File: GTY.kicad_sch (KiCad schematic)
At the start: 2 parts, among them J5 DF40HC(3.0)-120DS, U1 XCKU5P-FFVB676

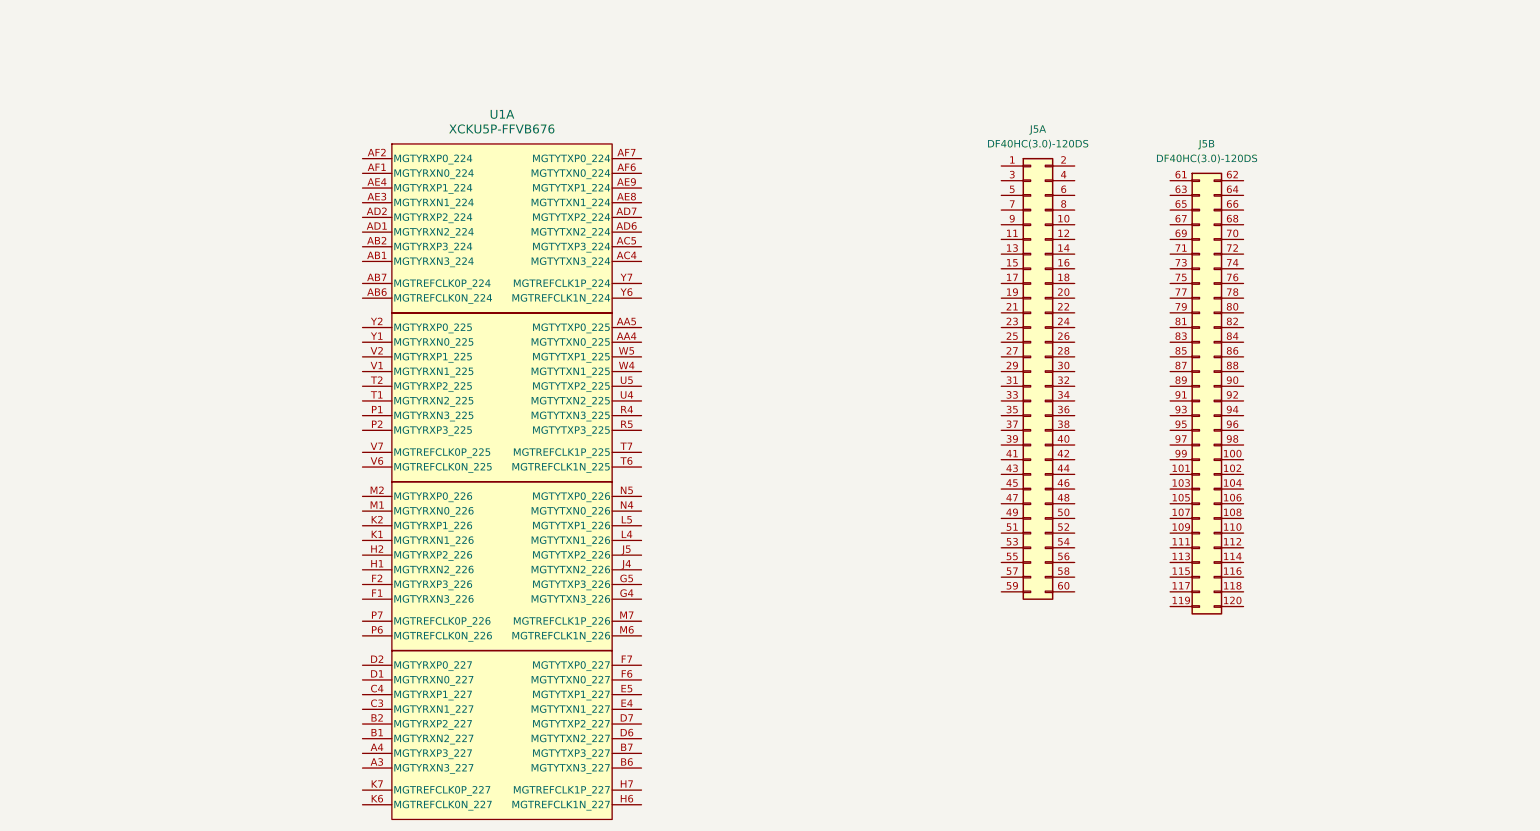
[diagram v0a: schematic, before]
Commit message: finishing schematic
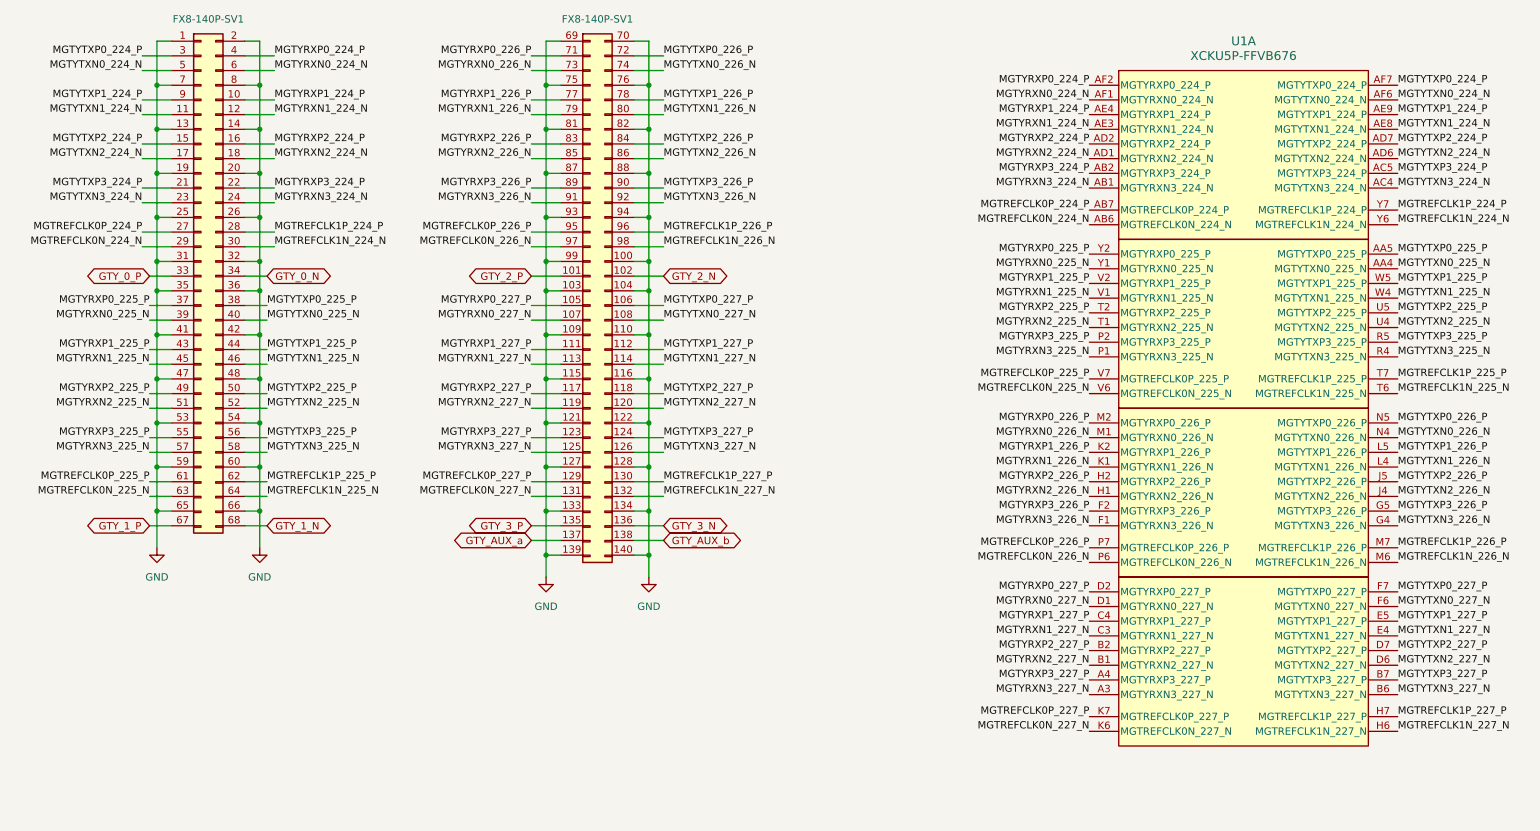
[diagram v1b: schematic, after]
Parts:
- J5: value DF40HC(3.0)-120DS -> FX8-140P-SV1; symbol dfdtc_Connector:Conn_02x60_Odd_Even -> dfdtc_Connector:Conn_02x70_Odd_Even
- J5: value DF40HC(3.0)-120DS -> FX8-140P-SV1; footprint Connector_Hirose_DF40:Hirose_DF40C-120DS-0.4V_2x60_P0.4mm -> Connector_Hirose_FX8:Hirose_FX8-140P-SV_2x70_P0.6mm; symbol dfdtc_Connector:Conn_02x60_Odd_Even -> dfdtc_Connector:Conn_02x70_Odd_Even
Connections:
- net GND: now reaches J5.100 (Pin_100)
- net GND: now also J5.1 (Pin_1), J5.103 (Pin_103), J5.104 (Pin_104), J5.109 (Pin_109), J5.110 (Pin_110), J5.115 (Pin_115), J5.116 (Pin_116), J5.121, J5.122, J5.127, J5.128, J5.13 (Pin_13), J5.133, J5.134, J5.139, J5.14 (Pin_14), J5.140, J5.19 (Pin_19), J5.2 (Pin_2), J5.20 (Pin_20), J5.25 (Pin_25), J5.26 (Pin_26), J5.31 (Pin_31), J5.32 (Pin_32), J5.35 (Pin_35), J5.36 (Pin_36), J5.41 (Pin_41), J5.42 (Pin_42), J5.47 (Pin_47), J5.48 (Pin_48), J5.53 (Pin_53), J5.54 (Pin_54), J5.59 (Pin_59), J5.60 (Pin_60), J5.65 (Pin_65), J5.66 (Pin_66), J5.69 (Pin_69), J5.7 (Pin_7), J5.70 (Pin_70), J5.75 (Pin_75), J5.76 (Pin_76), J5.8 (Pin_8), J5.81 (Pin_81), J5.82 (Pin_82), J5.87 (Pin_87), J5.88 (Pin_88), J5.93 (Pin_93), J5.94 (Pin_94), J5.99 (Pin_99)
- net GTY_2_P: now reaches J5.101 (Pin_101)
- net GTY_2_N: now reaches J5.102 (Pin_102)
- net MGTYRXP0_227_P: now reaches J5.105 (Pin_105)
- net MGTYRXP0_227_P: now also U1.D2 (MGTYRXP0_227_P)
- net MGTYTXP0_227_P: now reaches J5.106 (Pin_106)
- net MGTYTXP0_227_P: now also U1.F7 (MGTYTXP0_227_P)
- net MGTYRXN0_227_N: now reaches J5.107 (Pin_107)
- net MGTYRXN0_227_N: now also U1.D1 (MGTYRXN0_227_N)
- net MGTYTXN0_227_N: now reaches J5.108 (Pin_108)
- net MGTYTXN0_227_N: now also U1.F6 (MGTYTXN0_227_N)
- net MGTYRXP1_227_P: now reaches J5.111 (Pin_111)
- net MGTYRXP1_227_P: now also U1.C4 (MGTYRXP1_227_P)
- net MGTYTXP1_227_P: now reaches J5.112 (Pin_112)
- net MGTYTXP1_227_P: now also U1.E5 (MGTYTXP1_227_P)
- net MGTYRXN1_227_N: now reaches J5.113 (Pin_113)
- net MGTYRXN1_227_N: now also U1.C3 (MGTYRXN1_227_N)
- net MGTYTXN1_227_N: now reaches J5.114 (Pin_114)
- net MGTYTXN1_227_N: now also U1.E4 (MGTYTXN1_227_N)
- net MGTYRXP2_227_P: now reaches J5.117 (Pin_117)
- net MGTYRXP2_227_P: now also U1.B2 (MGTYRXP2_227_P)
- net MGTYTXP2_227_P: now reaches J5.118 (Pin_118)
- net MGTYTXP2_227_P: now also U1.D7 (MGTYTXP2_227_P)
- net MGTYRXN2_227_N: now reaches J5.119 (Pin_119)
- net MGTYRXN2_227_N: now also U1.B1 (MGTYRXN2_227_N)
- net MGTYTXN2_227_N: now reaches J5.120 (Pin_120)
- net MGTYTXN2_227_N: now also U1.D6 (MGTYTXN2_227_N)
- net MGTYRXP0_226_P: now reaches J5.71 (Pin_71)
- net MGTYRXP0_226_P: now also U1.M2 (MGTYRXP0_226_P)
- net MGTYTXP0_226_P: now reaches J5.72 (Pin_72)
- net MGTYTXP0_226_P: now also U1.N5 (MGTYTXP0_226_P)
- net MGTYRXN0_226_N: now reaches J5.73 (Pin_73)
- net MGTYRXN0_226_N: now also U1.M1 (MGTYRXN0_226_N)
- net MGTYTXN0_226_N: now reaches J5.74 (Pin_74)
- net MGTYTXN0_226_N: now also U1.N4 (MGTYTXN0_226_N)
- net MGTYRXP1_226_P: now reaches J5.77 (Pin_77)
- net MGTYRXP1_226_P: now also U1.K2 (MGTYRXP1_226_P)
- net MGTYTXP1_226_P: now reaches J5.78 (Pin_78)
- net MGTYTXP1_226_P: now also U1.L5 (MGTYTXP1_226_P)
- net MGTYRXN1_226_N: now reaches J5.79 (Pin_79)
- net MGTYRXN1_226_N: now also U1.K1 (MGTYRXN1_226_N)
- net MGTYTXN1_226_N: now reaches J5.80 (Pin_80)
- net MGTYTXN1_226_N: now also U1.L4 (MGTYTXN1_226_N)
- net MGTYRXP2_226_P: now reaches J5.83 (Pin_83)
- net MGTYRXP2_226_P: now also U1.H2 (MGTYRXP2_226_P)
- net MGTYTXP2_226_P: now reaches J5.84 (Pin_84)
- net MGTYTXP2_226_P: now also U1.J5 (MGTYTXP2_226_P)
- net MGTYRXN2_226_N: now reaches J5.85 (Pin_85)
- net MGTYRXN2_226_N: now also U1.H1 (MGTYRXN2_226_N)
- net MGTYTXN2_226_N: now reaches J5.86 (Pin_86)
- net MGTYTXN2_226_N: now also U1.J4 (MGTYTXN2_226_N)
- net MGTYRXP3_226_P: now reaches J5.89 (Pin_89)
- net MGTYRXP3_226_P: now also U1.F2 (MGTYRXP3_226_P)
- net MGTYTXP3_226_P: now reaches J5.90 (Pin_90)
- net MGTYTXP3_226_P: now also U1.G5 (MGTYTXP3_226_P)
- net MGTYRXN3_226_N: now reaches J5.91 (Pin_91)
- net MGTYRXN3_226_N: now also U1.F1 (MGTYRXN3_226_N)
- net MGTYTXN3_226_N: now reaches J5.92 (Pin_92)
- net MGTYTXN3_226_N: now also U1.G4 (MGTYTXN3_226_N)
- net MGTREFCLK0P_226_P: now reaches J5.95 (Pin_95)
- net MGTREFCLK0P_226_P: now also U1.P7 (MGTREFCLK0P_226_P)
- net MGTREFCLK1P_226_P: now reaches J5.96 (Pin_96)
- net MGTREFCLK1P_226_P: now also U1.M7 (MGTREFCLK1P_226_P)
- net MGTREFCLK0N_226_N: now reaches J5.97 (Pin_97)
- net MGTREFCLK0N_226_N: now also U1.P6 (MGTREFCLK0N_226_N)
- net MGTREFCLK1N_226_N: now reaches J5.98 (Pin_98)
- net MGTREFCLK1N_226_N: now also U1.M6 (MGTREFCLK1N_226_N)
- net MGTYRXP1_224_P: now reaches J5.10 (Pin_10)
- net MGTYRXP1_224_P: now also U1.AE4 (MGTYRXP1_224_P)
- net MGTYTXN1_224_N: now reaches J5.11 (Pin_11)
- net MGTYTXN1_224_N: now also U1.AE8 (MGTYTXN1_224_N)
- net MGTYRXN1_224_N: now reaches J5.12 (Pin_12)
- net MGTYRXN1_224_N: now also U1.AE3 (MGTYRXN1_224_N)
- net MGTYTXP2_224_P: now reaches J5.15 (Pin_15)
- net MGTYTXP2_224_P: now also U1.AD7 (MGTYTXP2_224_P)
- net MGTYRXP2_224_P: now reaches J5.16 (Pin_16)
- net MGTYRXP2_224_P: now also U1.AD2 (MGTYRXP2_224_P)
- net MGTYTXN2_224_N: now reaches J5.17 (Pin_17)
- net MGTYTXN2_224_N: now also U1.AD6 (MGTYTXN2_224_N)
- net MGTYRXN2_224_N: now reaches J5.18 (Pin_18)
- net MGTYRXN2_224_N: now also U1.AD1 (MGTYRXN2_224_N)
- net MGTYTXP3_224_P: now reaches J5.21 (Pin_21)
- net MGTYTXP3_224_P: now also U1.AC5 (MGTYTXP3_224_P)
- net MGTYRXP3_224_P: now reaches J5.22 (Pin_22)
- net MGTYRXP3_224_P: now also U1.AB2 (MGTYRXP3_224_P)
- net MGTYTXN3_224_N: now reaches J5.23 (Pin_23)
- net MGTYTXN3_224_N: now also U1.AC4 (MGTYTXN3_224_N)
- net MGTYRXN3_224_N: now reaches J5.24 (Pin_24)
- net MGTYRXN3_224_N: now also U1.AB1 (MGTYRXN3_224_N)
- net MGTREFCLK0P_224_P: now reaches J5.27 (Pin_27)
- net MGTREFCLK0P_224_P: now also U1.AB7 (MGTREFCLK0P_224_P)
- net MGTREFCLK1P_224_P: now reaches J5.28 (Pin_28)
- net MGTREFCLK1P_224_P: now also U1.Y7 (MGTREFCLK1P_224_P)
- net MGTREFCLK0N_224_N: now reaches J5.29 (Pin_29)
- net MGTREFCLK0N_224_N: now also U1.AB6 (MGTREFCLK0N_224_N)
- net MGTYTXP0_224_P: now reaches J5.3 (Pin_3)
- net MGTYTXP0_224_P: now also U1.AF7 (MGTYTXP0_224_P)
- net MGTREFCLK1N_224_N: now reaches J5.30 (Pin_30)
- net MGTREFCLK1N_224_N: now also U1.Y6 (MGTREFCLK1N_224_N)
- net GTY_0_P: now reaches J5.33 (Pin_33)
- net GTY_0_N: now reaches J5.34 (Pin_34)
- net MGTYRXP0_225_P: now reaches J5.37 (Pin_37)
- net MGTYRXP0_225_P: now also U1.Y2 (MGTYRXP0_225_P)
- net MGTYTXP0_225_P: now reaches J5.38 (Pin_38)
- net MGTYTXP0_225_P: now also U1.AA5 (MGTYTXP0_225_P)
- net MGTYRXN0_225_N: now reaches J5.39 (Pin_39)
- net MGTYRXN0_225_N: now also U1.Y1 (MGTYRXN0_225_N)
- net MGTYRXP0_224_P: now reaches J5.4 (Pin_4)
- net MGTYRXP0_224_P: now also U1.AF2 (MGTYRXP0_224_P)
- net MGTYTXN0_225_N: now reaches J5.40 (Pin_40)
- net MGTYTXN0_225_N: now also U1.AA4 (MGTYTXN0_225_N)
- net MGTYRXP1_225_P: now reaches J5.43 (Pin_43)
- net MGTYRXP1_225_P: now also U1.V2 (MGTYRXP1_225_P)
- net MGTYTXP1_225_P: now reaches J5.44 (Pin_44)
- net MGTYTXP1_225_P: now also U1.W5 (MGTYTXP1_225_P)
- net MGTYRXN1_225_N: now reaches J5.45 (Pin_45)
- net MGTYRXN1_225_N: now also U1.V1 (MGTYRXN1_225_N)
- net MGTYTXN1_225_N: now reaches J5.46 (Pin_46)
- net MGTYTXN1_225_N: now also U1.W4 (MGTYTXN1_225_N)
- net MGTYRXP2_225_P: now reaches J5.49 (Pin_49)
- net MGTYRXP2_225_P: now also U1.T2 (MGTYRXP2_225_P)
- net MGTYTXN0_224_N: now reaches J5.5 (Pin_5)
- net MGTYTXN0_224_N: now also U1.AF6 (MGTYTXN0_224_N)
- net MGTYTXP2_225_P: now reaches J5.50 (Pin_50)
- net MGTYTXP2_225_P: now also U1.U5 (MGTYTXP2_225_P)
- net MGTYRXN2_225_N: now reaches J5.51 (Pin_51)
- net MGTYRXN2_225_N: now also U1.T1 (MGTYRXN2_225_N)
- net MGTYTXN2_225_N: now reaches J5.52 (Pin_52)
- net MGTYTXN2_225_N: now also U1.U4 (MGTYTXN2_225_N)
- net MGTYRXP3_225_P: now reaches J5.55 (Pin_55)
- net MGTYRXP3_225_P: now also U1.P2 (MGTYRXP3_225_P)
- net MGTYTXP3_225_P: now reaches J5.56 (Pin_56)
- net MGTYTXP3_225_P: now also U1.R5 (MGTYTXP3_225_P)
- net MGTYRXN3_225_N: now reaches J5.57 (Pin_57)
- net MGTYRXN3_225_N: now also U1.P1 (MGTYRXN3_225_N)
- net MGTYTXN3_225_N: now reaches J5.58 (Pin_58)
- net MGTYTXN3_225_N: now also U1.R4 (MGTYTXN3_225_N)
- net MGTYRXN0_224_N: now reaches J5.6 (Pin_6)
- net MGTYRXN0_224_N: now also U1.AF1 (MGTYRXN0_224_N)
- net MGTYTXP1_224_P: now reaches J5.9 (Pin_9)
- net MGTYTXP1_224_P: now also U1.AE9 (MGTYTXP1_224_P)
- net MGTYRXN3_227_N: now reaches U1.A3 (MGTYRXN3_227_N)
- net MGTYRXN3_227_N: now also J5.125
- net MGTYRXP3_227_P: now reaches U1.A4 (MGTYRXP3_227_P)
- net MGTYRXP3_227_P: now also J5.123
- net MGTYTXN3_227_N: now reaches U1.B6 (MGTYTXN3_227_N)
- net MGTYTXN3_227_N: now also J5.126
- net MGTYTXP3_227_P: now reaches U1.B7 (MGTYTXP3_227_P)
- net MGTYTXP3_227_P: now also J5.124
- net MGTREFCLK1N_227_N: now reaches U1.H6 (MGTREFCLK1N_227_N)
- net MGTREFCLK1N_227_N: now also J5.132
- net MGTREFCLK1P_227_P: now reaches U1.H7 (MGTREFCLK1P_227_P)
- net MGTREFCLK1P_227_P: now also J5.130
- net MGTREFCLK0N_227_N: now reaches U1.K6 (MGTREFCLK0N_227_N)
- net MGTREFCLK0N_227_N: now also J5.131
- net MGTREFCLK0P_227_P: now reaches U1.K7 (MGTREFCLK0P_227_P)
- net MGTREFCLK0P_227_P: now also J5.129
- net MGTREFCLK1N_225_N: now reaches U1.T6 (MGTREFCLK1N_225_N)
- net MGTREFCLK1N_225_N: now also J5.64 (Pin_64)
- net MGTREFCLK1P_225_P: now reaches U1.T7 (MGTREFCLK1P_225_P)
- net MGTREFCLK1P_225_P: now also J5.62 (Pin_62)
- net MGTREFCLK0N_225_N: now reaches U1.V6 (MGTREFCLK0N_225_N)
- net MGTREFCLK0N_225_N: now also J5.63 (Pin_63)
- net MGTREFCLK0P_225_P: now reaches U1.V7 (MGTREFCLK0P_225_P)
- net MGTREFCLK0P_225_P: now also J5.61 (Pin_61)
- new net GTY_1_N: J5.68 (Pin_68)
- new net GTY_1_P: J5.67 (Pin_67)
- new net GTY_3_N: J5.136
- new net GTY_3_P: J5.135
- new net GTY_AUX_a: J5.137
- new net GTY_AUX_b: J5.138
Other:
- moved on the sheet: U1A
